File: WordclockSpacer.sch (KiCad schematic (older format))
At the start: 133 parts, among them J1 Input, J10 LED1, J11 LED7, J12 LED2Back, J13 LED2, J14 LED5, J15 LED8, J16 LED6, J17 Conn_01x03_Female, J18 LED1, J19 LED7, J2 Conn_01x02_Male, J20 LED2, J21 LED5, J22 LED8, J23 LED6, J24 LED9, J25 LED1, J26 LED7, J27 LED2, J28 LED5, J29 LED8, J3 Conn_01x02_Male, J30 LED6, J31 LED9, J32 Conn_01x10, J33 Conn_01x10, J34 LED4, J35 LED4, J36 Conn_02x04_Odd_Even, J37 Conn_01x03_Female, J38 LED_OUT, J39 LED_IN, J4 Output, J40 LED_IN, J5 Middle Out, J6 Back Line In, J7 Back Line Out middle, J8 Back Line Out, J9 LED1Back, SW1 SW_Push, U1 ESP-12E, U2 74HCT1G125GW

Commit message: improved footprint
Signed-off-by: Empire
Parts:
- C1, C10, C11, C12, C15, C16, C17, C18, C19, C2, C20, C21, C22, C23, C24, C25, C26, C27, C28, C29, C3, C30, C31, C32, C33, C34, C35, C36, C37, C38, C39, C4, C40, C41, C42, C45, C5, C6, C7, C8, C9: footprint Capacitor_SMD:C_1206_3216Metric -> (none)
- C13, C14, C43, C44: footprint Capacitor_THT:CP_Radial_D6.3mm_P2.50mm -> (none)
- D1, D10, D11, D12, D13, D14, D15, D16, D17, D18, D19, D2, D20, D21, D22, D23, D24, D25, D26, D27, D28, D29, D3, D30, D31, D32, D33, D34, D35, D36, D37, D38, D39, D4, D40, D5, D6, D7, D8, D9: footprint LED_SMD:LED_WS2812B_PLCC4_5.0x5.0mm_P3.2mm -> Wordclock:LED_WS2812B_PLCC4_5.0x5.0mm_P3.2mmMitEcke
- J1: footprint Connector_PinSocket_2.54mm:PinSocket_1x07_P2.54mm_Horizontal -> (none)
- J10, J11, J12, J13, J14, J15, J16, J18, J19, J20, J21, J22, J23, J24, J25, J26, J27, J28, J29, J30, J31, J34, J35, J38, J39, J40, J9: footprint Connector_PinHeader_2.54mm:PinHeader_1x01_P2.54mm_Vertical -> (none)
- J17, J37: footprint Connector_PinSocket_2.54mm:PinSocket_1x03_P2.54mm_Vertical -> (none)
- J2, J3: footprint Connector_Wire:SolderWirePad_1x02_P3.81mm_Drill1.2mm -> (none)
- J32, J33: footprint Connector_PinSocket_2.54mm:PinSocket_1x10_P2.54mm_Vertical -> (none)
- J36: footprint Connector_PinHeader_2.54mm:PinHeader_2x04_P2.54mm_Vertical -> (none)
- J4, J5: footprint Connector_PinHeader_2.54mm:PinHeader_1x07_P2.54mm_Horizontal -> (none)
- J6: footprint Connector_PinSocket_2.54mm:PinSocket_1x03_P2.54mm_Horizontal -> (none)
- J7, J8: footprint Connector_PinHeader_2.54mm:PinHeader_1x03_P2.54mm_Horizontal -> (none)
- R1, R2, R3, R4, R5: footprint Resistor_SMD:R_0805_2012Metric -> (none)
- SW1: footprint Button_Switch_SMD:SW_SPST_B3S-1000 -> (none)
- U2: footprint 74HCT1G125GW:SOT65P210X110-5N -> SOT65P210X110-5N

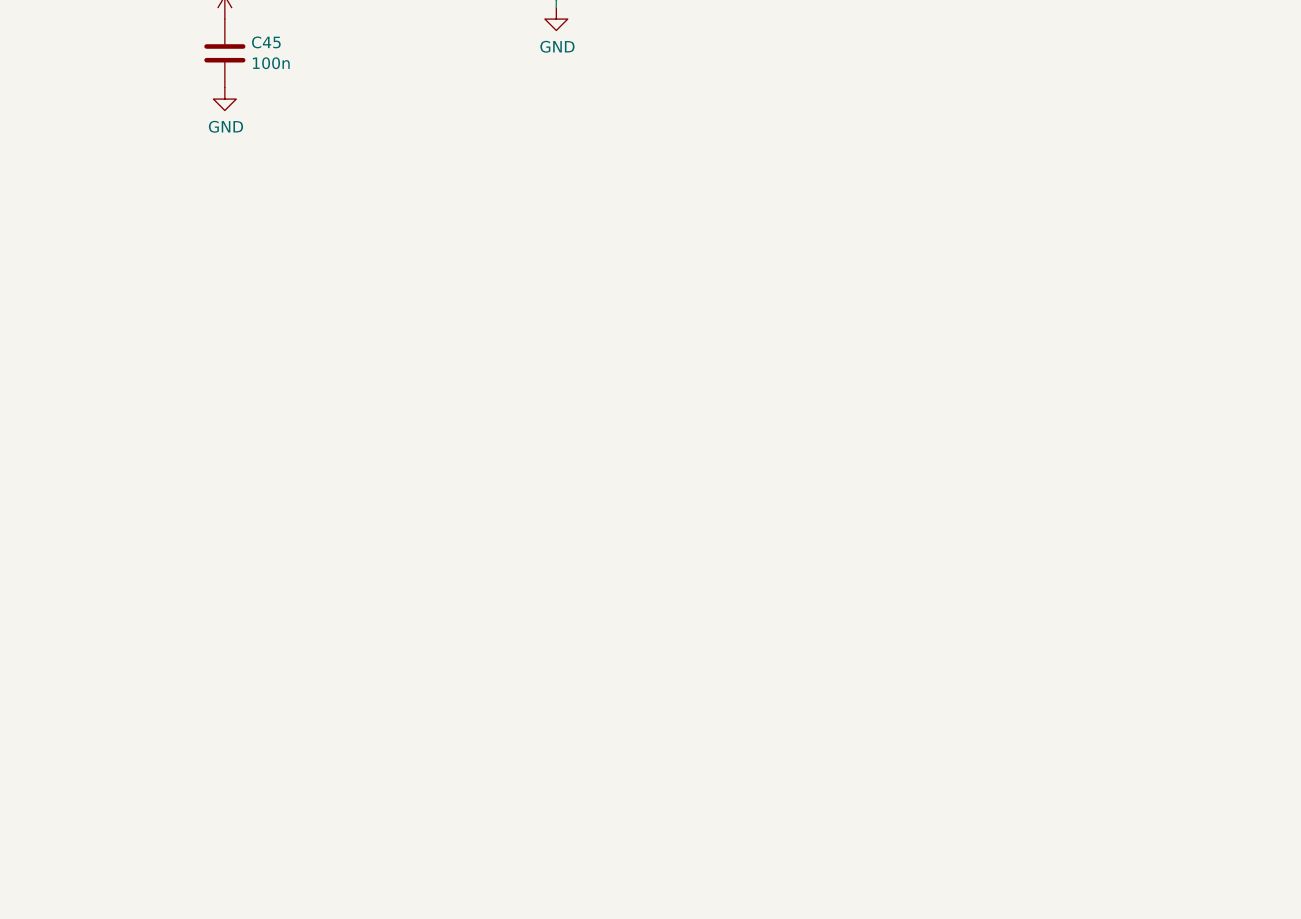
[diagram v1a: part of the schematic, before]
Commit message: V3 Alpha
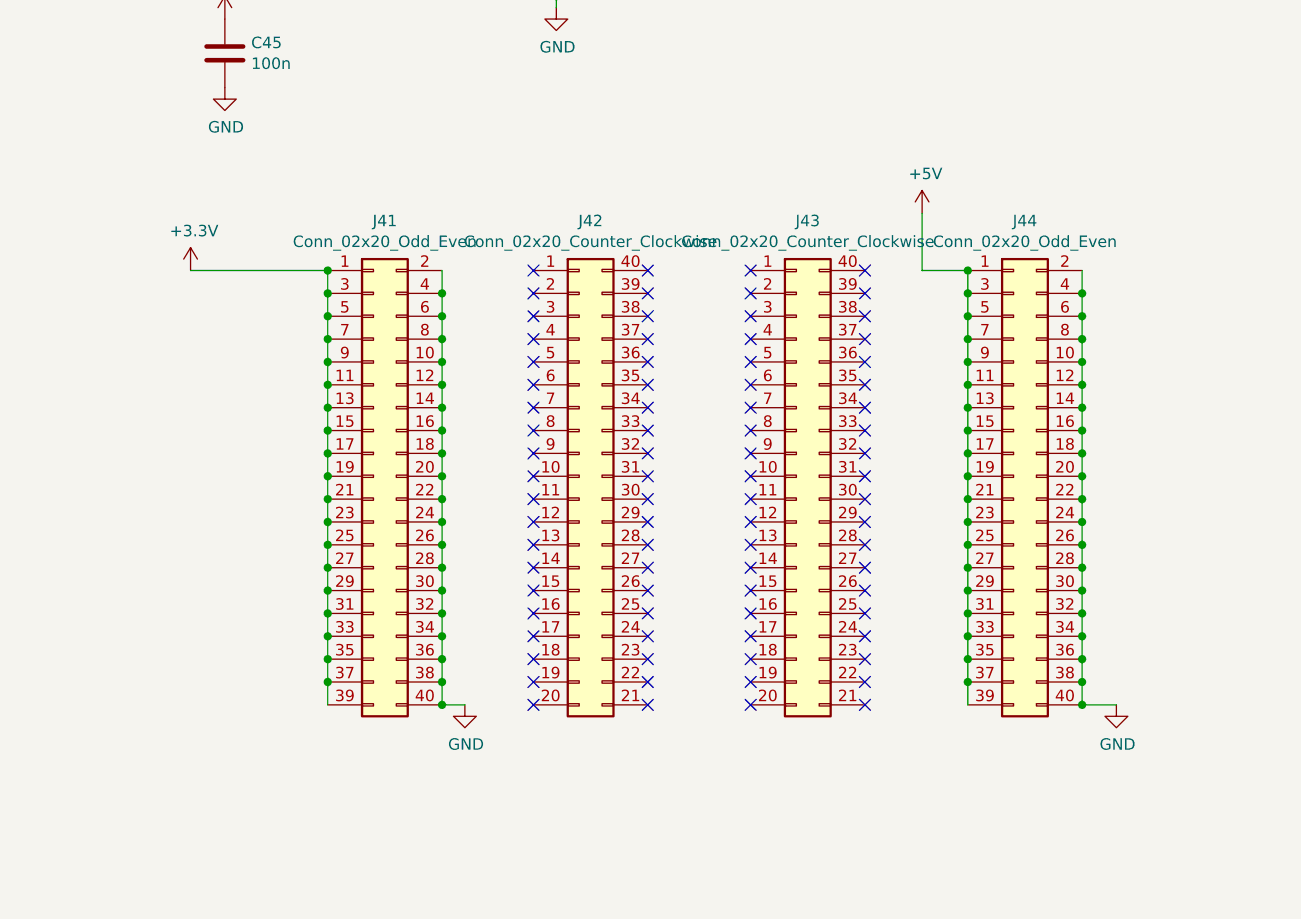
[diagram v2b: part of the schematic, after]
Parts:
- added J41, J44: Conn_02x20_Odd_Even, Connector_PinSocket_2.54mm:PinSocket_2x20_P2.54mm_Vertical, symbol Connector_Generic:Conn_02x20_Odd_Even
- added J42, J43: Conn_02x20_Counter_Clockwise, Connector_PinSocket_2.54mm:PinSocket_2x20_P2.54mm_Vertical, symbol Connector_Generic:Conn_02x20_Counter_Clockwise
- C1, C10, C11, C12, C15, C16, C17, C18, C19, C2, C20, C21, C22, C23, C24, C25, C26, C27, C28, C29, C3, C30, C31, C32, C33, C34, C35, C36, C37, C38, C39, C4, C40, C41, C42, C45, C5, C6, C7, C8, C9: footprint (none) -> Capacitor_SMD:C_0805_2012Metric_Pad1.15x1.40mm_HandSolder
- C13, C14, C43, C44: footprint (none) -> Capacitor_THT:CP_Radial_D6.3mm_P2.50mm
- J1: footprint (none) -> Connector_PinHeader_2.54mm:PinHeader_1x07_P2.54mm_Vertical
- J10, J11, J12, J13, J14, J15, J16, J18, J19, J20, J21, J22, J23, J24, J25, J26, J27, J28, J29, J30, J31, J34, J35, J9: footprint (none) -> Connector_PinHeader_2.54mm:PinHeader_1x01_P2.54mm_Vertical
- J17, J6, J7, J8: footprint (none) -> Connector_PinSocket_2.54mm:PinSocket_1x03_P2.54mm_Horizontal
- J2, J3: footprint (none) -> Connector_Wire:SolderWirePad_1x02_P3.81mm_Drill1.2mm
- J32, J33: footprint (none) -> Connector_PinSocket_2.54mm:PinSocket_1x10_P2.54mm_Vertical
- J36: footprint (none) -> Connector_PinSocket_2.54mm:PinSocket_2x04_P2.54mm_Vertical
- J37: footprint (none) -> Connector_PinSocket_2.54mm:PinSocket_1x03_P2.54mm_Vertical
- J38, J39, J40: footprint (none) -> Connector_PinSocket_2.54mm:PinSocket_1x01_P2.54mm_Horizontal
- J4, J5: footprint (none) -> Connector_PinSocket_2.54mm:PinSocket_1x07_P2.54mm_Horizontal
- R1, R2, R3, R4, R5: footprint (none) -> Resistor_SMD:R_0805_2012Metric_Pad1.15x1.40mm_HandSolder
- SW1: footprint (none) -> Button_Switch_SMD:SW_SPST_B3S-1000
- U2: footprint SOT65P210X110-5N -> 74HCT1G125GW:SOT65P210X110-5N
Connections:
- net +3V3: now also J41.1 (Pin_1), J41.11 (Pin_11), J41.13 (Pin_13), J41.15 (Pin_15), J41.17 (Pin_17), J41.19 (Pin_19), J41.21 (Pin_21), J41.23 (Pin_23), J41.25 (Pin_25), J41.27 (Pin_27), J41.29 (Pin_29), J41.3 (Pin_3), J41.31 (Pin_31), J41.33 (Pin_33), J41.35 (Pin_35), J41.37 (Pin_37), J41.39 (Pin_39), J41.5 (Pin_5), J41.7 (Pin_7), J41.9 (Pin_9)
- net +5V: now also J44.1 (Pin_1), J44.11 (Pin_11), J44.13 (Pin_13), J44.15 (Pin_15), J44.17 (Pin_17), J44.19 (Pin_19), J44.21 (Pin_21), J44.23 (Pin_23), J44.25 (Pin_25), J44.27 (Pin_27), J44.29 (Pin_29), J44.3 (Pin_3), J44.31 (Pin_31), J44.33 (Pin_33), J44.35 (Pin_35), J44.37 (Pin_37), J44.39 (Pin_39), J44.5 (Pin_5), J44.7 (Pin_7), J44.9 (Pin_9)
- net GND: now also J41.10 (Pin_10), J41.12 (Pin_12), J41.14 (Pin_14), J41.16 (Pin_16), J41.18 (Pin_18), J41.2 (Pin_2), J41.20 (Pin_20), J41.22 (Pin_22), J41.24 (Pin_24), J41.26 (Pin_26), J41.28 (Pin_28), J41.30 (Pin_30), J41.32 (Pin_32), J41.34 (Pin_34), J41.36 (Pin_36), J41.38 (Pin_38), J41.4 (Pin_4), J41.40 (Pin_40), J41.6 (Pin_6), J41.8 (Pin_8), J44.10 (Pin_10), J44.12 (Pin_12), J44.14 (Pin_14), J44.16 (Pin_16), J44.18 (Pin_18), J44.2 (Pin_2), J44.20 (Pin_20), J44.22 (Pin_22), J44.24 (Pin_24), J44.26 (Pin_26), J44.28 (Pin_28), J44.30 (Pin_30), J44.32 (Pin_32), J44.34 (Pin_34), J44.36 (Pin_36), J44.38 (Pin_38), J44.4 (Pin_4), J44.40 (Pin_40), J44.6 (Pin_6), J44.8 (Pin_8)
- no-connect marks 0 -> 80

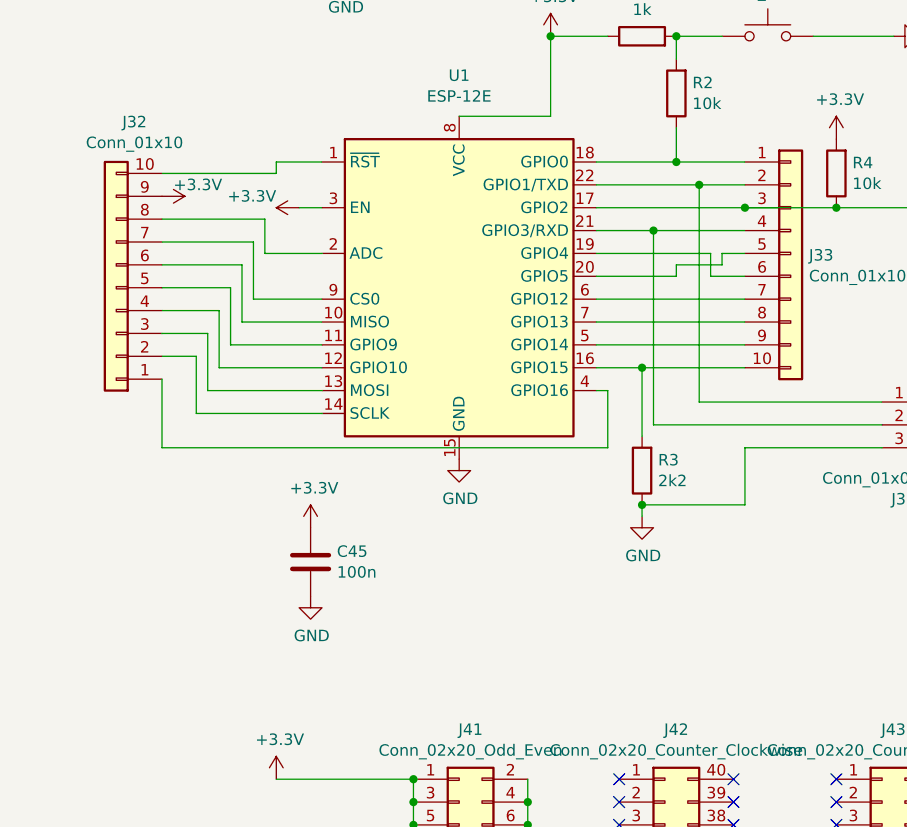
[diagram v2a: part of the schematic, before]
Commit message: no Alpha. it is V3
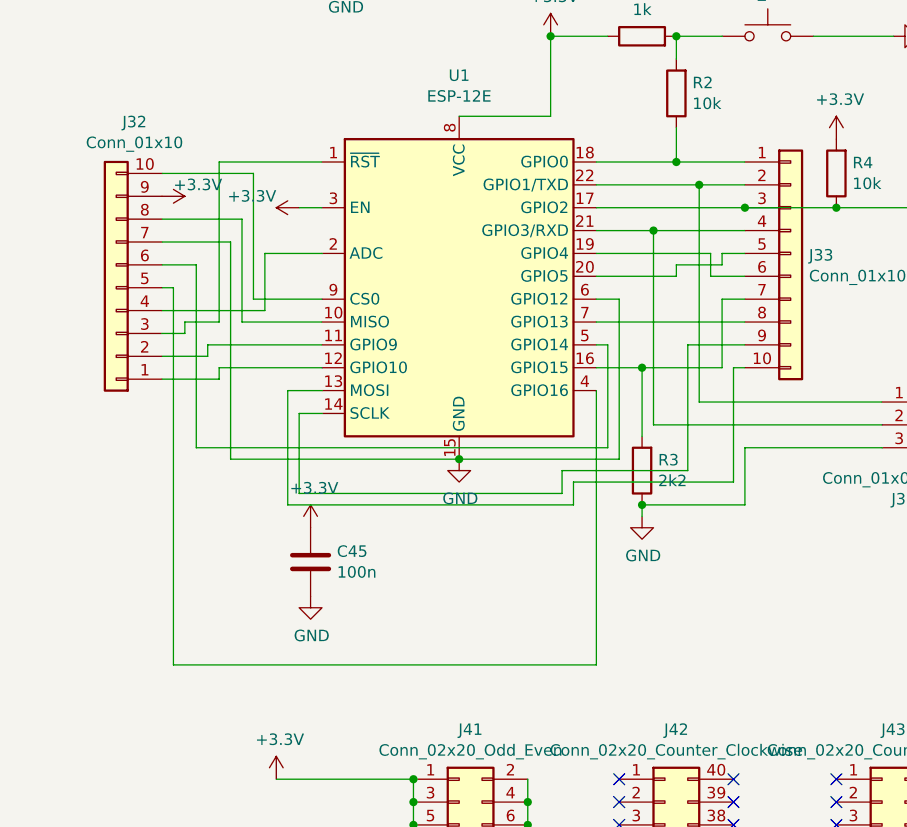
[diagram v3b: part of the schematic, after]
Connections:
- net GND: now also J32.7 (Pin_7), U1.6 (GPIO12)
- net at U1.1 (~RST): now also J32.3 (Pin_3); no longer J32.10 (Pin_10)
- net at U1.10 (MISO): now also J32.8 (Pin_8); no longer J32.6 (Pin_6)
- net at U1.11 (GPIO9): now also J32.2 (Pin_2); no longer J32.5 (Pin_5)
- net at U1.12 (GPIO10): now also J32.1 (Pin_1); no longer J32.4 (Pin_4)
- net at U1.13 (MOSI): now also J33.10 (Pin_10); no longer J32.3 (Pin_3)
- net at U1.14 (SCLK): now also J33.9 (Pin_9); no longer J32.2 (Pin_2)
- net at R3.2, U1.16 (GPIO15): now also J33.7 (Pin_7); no longer J33.10 (Pin_10)
- net at U1.2 (ADC): now also J32.4 (Pin_4); no longer J32.8 (Pin_8)
- net at U1.4 (GPIO16): now also J32.5 (Pin_5); no longer J32.1 (Pin_1)
- net at U1.5 (GPIO14): now also J32.6 (Pin_6); no longer J33.9 (Pin_9)
- net at U1.9 (CS0): now also J32.10 (Pin_10); no longer J32.7 (Pin_7)
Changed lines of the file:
@@
 	5750 3450 6000 3450
 Wire Wire Line
-	5750 3750 6400 3750
-Wire Wire Line
 	5750 3850 6400 3850
 Wire Wire Line
-	5750 3950 6400 3950
-Wire Wire Line
-	4550 3150 4350 3150
-Wire Wire Line
 	4550 3750 4250 3750
 Wire Wire Line
 	4200 3850 4550 3850
 Wire Wire Line
-	4150 3700 4150 3950
-Wire Wire Line
-	4150 3950 4550 3950
-Wire Wire Line
-	4550 4050 4100 4050
-Wire Wire Line
-	4100 4050 4100 3800
-Wire Wire Line
-	4550 4150 4050 4150
-Wire Wire Line
-	4050 4150 4050 3900
-Wire Wire Line
-	4050 3900 3850 3900
-Wire Wire Line
-	3850 4000 4000 4000
-Wire Wire Line
-	4000 4000 4000 4250
-Wire Wire Line
-	4000 4250 4550 4250
-Wire Wire Line
-	3850 3800 4100 3800
-Wire Wire Line
-	3850 3700 4150 3700
-Wire Wire Line
 	4300 3550 4550 3550
-Wire Wire Line
-	4200 3600 4200 3850
-Wire Wire Line
-	3850 3600 4200 3600
-Wire Wire Line
-	4250 3750 4250 3500
-Wire Wire Line
-	3850 3500 4250 3500
-Wire Wire Line
-	4300 3550 4300 3400
-Wire Wire Line
-	3850 3400 4300 3400
-Wire Wire Line
-	3850 3200 4350 3200
-Wire Wire Line
-	4350 3200 4350 3150
 $Comp
 L power:+3.3V #PWR0128
@@
 	0    1    1    0
 $EndComp
-Wire Wire Line
-	3850 4100 3850 4400
 $Comp
 L power:PWR_FLAG #FLG0101
@@
 	1    0    0    -1
 $EndComp
-Connection ~ 5950 4050
 Wire Wire Line
 	5950 4050 5750 4050
-Wire Wire Line
-	5950 4050 6400 4050
-Wire Wire Line
-	5750 4150 5800 4150
-Wire Wire Line
-	5800 4150 5800 4400
-Wire Wire Line
-	5800 4400 3850 4400
 Wire Wire Line
 	7000 4200 6200 4200
@@
 Wire Wire Line
 	5450 7650 5450 7550
+Wire Wire Line
+	5750 4150 5750 5350
+Wire Wire Line
+	4300 3550 4300 3800
+Wire Wire Line
+	4300 3800 3850 3800
+Wire Wire Line
+	4550 3150 4100 3150
+Wire Wire Line
+	4200 3400 3850 3400
+Wire Wire Line
+	4200 3400 4200 3850
+Wire Wire Line
+	3850 3200 4250 3200
+Wire Wire Line
+	4250 3200 4250 3750
+Wire Wire Line
+	4100 4050 4550 4050
+Wire Wire Line
+	3850 3900 3950 3900
+Wire Wire Line
+	3950 3900 3950 3850
+Wire Wire Line
+	3950 3850 4100 3850
+Wire Wire Line
+	4100 3150 4100 3850
+Wire Wire Line
+	3850 3700 3900 3700
+Wire Wire Line
+	3900 3700 3900 5350
+Wire Wire Line
+	3900 5350 5750 5350
+Wire Wire Line
+	5950 4050 6300 4050
+Wire Wire Line
+	6300 4050 6300 3750
+Wire Wire Line
+	6300 3750 6400 3750
+Connection ~ 5950 4050
+Wire Wire Line
+	4550 4250 4450 4250
+Wire Wire Line
+	4450 4250 4450 4600
+Wire Wire Line
+	4450 4600 5600 4600
+Wire Wire Line
+	5600 4600 5600 4500
+Wire Wire Line
+	5600 4500 6150 4500
+Wire Wire Line
+	6150 4500 6150 3950
+Wire Wire Line
+	6150 3950 6400 3950
+Wire Wire Line
+	4550 4150 4400 4150
+Wire Wire Line
+	4400 4150 4400 4650
+Wire Wire Line
+	4400 4650 5650 4650
+Wire Wire Line
+	5650 4650 5650 4550
+Wire Wire Line
+	5650 4550 6350 4550
+Wire Wire Line
+	6350 4550 6350 4050
+Wire Wire Line
+	6350 4050 6400 4050
+Wire Wire Line
+	4100 4050 4100 4100
+Wire Wire Line
+	4100 4100 3850 4100
+Wire Wire Line
+	4050 3950 4050 4000
+Wire Wire Line
+	4050 4000 3850 4000
+Wire Wire Line
+	4050 3950 4550 3950
+Wire Wire Line
+	5750 3950 5800 3950
+Wire Wire Line
+	5800 3950 5800 4400
+Wire Wire Line
+	5800 4400 4000 4400
+Wire Wire Line
+	4000 4400 4000 3600
+Wire Wire Line
+	4000 3600 3850 3600
+Wire Wire Line
+	5750 3750 5850 3750
+Wire Wire Line
+	5850 3750 5850 4450
+Wire Wire Line
+	5850 4450 5150 4450
+Wire Wire Line
+	4150 4450 4150 3500
+Wire Wire Line
+	4150 3500 3850 3500
+Connection ~ 5150 4450
+Wire Wire Line
+	5150 4450 4150 4450
 $EndSCHEMATC

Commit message: V3.0 added AMS1117
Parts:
- C13, C14, C43, C44: symbol Device:CP -> WordclockSpacer-rescue:CP-Device
- U2: symbol 74HCT1G125GW:74HCT1G125GW -> WordclockSpacer-rescue:74HCT1G125GW-74HCT1G125GW
